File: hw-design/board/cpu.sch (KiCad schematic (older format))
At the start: 23 parts, among them P1 CHAIN, P2 USB_OTG, P3 SWD, Q7 BC857, SW1 SW_PUSH, U4 LPC11U24FBD48/401, Y1 12MHz

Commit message: sch: DRC checked
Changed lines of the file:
@@
 $EndDescr
 $Comp
-L GNDD #PWR52
+L GNDD #PWR045
 U 1 1 54E5DFA7
 P 9200 4250
-F 0 "#PWR52" H 9200 4000 60  0001 C CNN
+F 0 "#PWR045" H 9200 4000 60  0001 C CNN
 F 1 "GNDD" H 9200 4100 60  0000 C CNN
 F 2 "" H 9200 4250 60  0000 C CNN
@@
 $EndComp
 $Comp
-L GNDD #PWR43
+L GNDD #PWR046
 U 1 1 556F6417
 P 3300 4600
-F 0 "#PWR43" H 3300 4350 50  0001 C CNN
+F 0 "#PWR046" H 3300 4350 50  0001 C CNN
 F 1 "GNDD" H 3300 4450 50  0000 C CNN
 F 2 "" H 3300 4600 60  0000 C CNN
@@
 $EndComp
 $Comp
-L GNDD #PWR44
+L GNDD #PWR047
 U 1 1 556F65EC
 P 3550 4600
-F 0 "#PWR44" H 3550 4350 50  0001 C CNN
+F 0 "#PWR047" H 3550 4350 50  0001 C CNN
 F 1 "GNDD" H 3550 4450 50  0000 C CNN
 F 2 "" H 3550 4600 60  0000 C CNN
@@
 $EndComp
 $Comp
-L +3.3V #PWR49
+L +3.3V #PWR048
 U 1 1 55705A80
 P 5900 850
-F 0 "#PWR49" H 5900 700 50  0001 C CNN
+F 0 "#PWR048" H 5900 700 50  0001 C CNN
 F 1 "+3.3V" H 5900 990 50  0000 C CNN
 F 2 "" H 5900 850 60  0000 C CNN
@@
 $EndComp
 $Comp
-L GNDD #PWR48
+L GNDD #PWR049
 U 1 1 557DC875
 P 5600 1450
-F 0 "#PWR48" H 5600 1200 50  0001 C CNN
+F 0 "#PWR049" H 5600 1200 50  0001 C CNN
 F 1 "GNDD" H 5600 1300 50  0000 C CNN
 F 2 "" H 5600 1450 60  0000 C CNN
@@
 $EndComp
 $Comp
-L GNDD #PWR51
+L GNDD #PWR050
 U 1 1 557DCAD9
 P 6200 1450
-F 0 "#PWR51" H 6200 1200 50  0001 C CNN
+F 0 "#PWR050" H 6200 1200 50  0001 C CNN
 F 1 "GNDD" H 6200 1300 50  0000 C CNN
 F 2 "" H 6200 1450 60  0000 C CNN
@@
 $EndComp
 $Comp
-L GNDD #PWR50
+L GNDD #PWR051
 U 1 1 557DD01E
 P 5900 4750
-F 0 "#PWR50" H 5900 4500 50  0001 C CNN
+F 0 "#PWR051" H 5900 4500 50  0001 C CNN
 F 1 "GNDD" H 5900 4600 50  0000 C CNN
 F 2 "" H 5900 4750 60  0000 C CNN
@@
 $EndComp
 $Comp
-L GNDD #PWR42
+L GNDD #PWR052
 U 1 1 557DE7E3
 P 2850 6600
-F 0 "#PWR42" H 2850 6350 50  0001 C CNN
+F 0 "#PWR052" H 2850 6350 50  0001 C CNN
 F 1 "GNDD" H 2850 6450 50  0000 C CNN
 F 2 "" H 2850 6600 60  0000 C CNN
@@
 $EndComp
 $Comp
-L VCC #PWR45
+L VCC #PWR053
 U 1 1 557DE7F0
 P 3750 6300
-F 0 "#PWR45" H 3750 6150 50  0001 C CNN
+F 0 "#PWR053" H 3750 6150 50  0001 C CNN
 F 1 "VCC" H 3750 6450 50  0000 C CNN
 F 2 "" H 3750 6300 60  0000 C CNN
@@
 $EndComp
 $Comp
-L +3.3V #PWR41
+L +3.3V #PWR054
 U 1 1 557E22DB
 P 2050 6500
-F 0 "#PWR41" H 2050 6350 50  0001 C CNN
+F 0 "#PWR054" H 2050 6350 50  0001 C CNN
 F 1 "+3.3V" H 2050 6640 50  0000 C CNN
 F 2 "" H 2050 6500 60  0000 C CNN
@@
 $EndComp
 $Comp
-L GNDD #PWR46
+L GNDD #PWR055
 U 1 1 557EA320
 P 3750 6900
-F 0 "#PWR46" H 3750 6650 50  0001 C CNN
+F 0 "#PWR055" H 3750 6650 50  0001 C CNN
 F 1 "GNDD" H 3750 6750 50  0000 C CNN
 F 2 "" H 3750 6900 60  0000 C CNN
@@
 $EndComp
 $Comp
-L GNDD #PWR40
+L GNDD #PWR056
 U 1 1 557F3440
 P 1700 1450
-F 0 "#PWR40" H 1700 1200 50  0001 C CNN
+F 0 "#PWR056" H 1700 1200 50  0001 C CNN
 F 1 "GNDD" H 1700 1300 50  0000 C CNN
 F 2 "" H 1700 1450 60  0000 C CNN
@@
 $EndComp
 $Comp
-L +3.3V #PWR54
+L +3.3V #PWR057
 U 1 1 55802FA1
 P 10000 1250
-F 0 "#PWR54" H 10000 1100 50  0001 C CNN
+F 0 "#PWR057" H 10000 1100 50  0001 C CNN
 F 1 "+3.3V" H 10000 1390 50  0000 C CNN
 F 2 "" H 10000 1250 60  0000 C CNN
@@
 $EndComp
 $Comp
-L GNDD #PWR55
+L GNDD #PWR058
 U 1 1 55803C49
 P 10000 2250
-F 0 "#PWR55" H 10000 2000 50  0001 C CNN
+F 0 "#PWR058" H 10000 2000 50  0001 C CNN
 F 1 "GNDD" H 10000 2100 50  0000 C CNN
 F 2 "" H 10000 2250 60  0000 C CNN
@@
 $EndComp
 $Comp
-L GNDD #PWR53
+L GNDD #PWR059
 U 1 1 55806665
 P 9600 2550
-F 0 "#PWR53" H 9600 2300 50  0001 C CNN
+F 0 "#PWR059" H 9600 2300 50  0001 C CNN
 F 1 "GNDD" H 9600 2400 50  0000 C CNN
 F 2 "" H 9600 2550 60  0000 C CNN
@@
 LCD_CONTRAST
 Wire Wire Line
-	9200 3850 9200 3950
-Wire Wire Line
-	9200 3950 9200 4150
-Wire Wire Line
-	9200 4150 9200 4250
+	9200 3850 9200 4250
 Wire Wire Line
 	9900 4150 10100 4150
@@
 	4050 4100 4050 4200
 Wire Wire Line
-	4050 4200 3850 4200
-Wire Wire Line
-	3850 4200 3550 4200
+	4050 4200 3550 4200
 Wire Wire Line
 	3550 4200 3550 4250
@@
 	3300 4250 3300 3900
 Wire Wire Line
-	3300 3900 3850 3900
-Wire Wire Line
-	3850 3900 4050 3900
+	3300 3900 4050 3900
 Wire Wire Line
 	4050 3900 4050 4000
@@
 	5800 1600 5800 900
 Wire Wire Line
-	5600 900  5800 900
-Wire Wire Line
-	5800 900  5900 900
-Wire Wire Line
-	5900 900  6000 900
-Wire Wire Line
-	6000 900  6200 900
+	5600 900  6200 900
 Wire Wire Line
 	6000 900  6000 1600
@@
 	5800 4600 5800 4700
 Wire Wire Line
-	5800 4700 5900 4700
-Wire Wire Line
-	5900 4700 6000 4700
+	5800 4700 6000 4700
 Wire Wire Line
 	6000 4700 6000 4600
@@
 	3450 7200 3450 6400
 Wire Wire Line
-	4200 6450 4350 6450
-Wire Wire Line
-	4350 6450 4500 6450
-Wire Wire Line
-	3550 6450 3750 6450
-Wire Wire Line
-	3750 6450 3900 6450
+	4200 6450 4500 6450
+Wire Wire Line
+	3550 6450 3900 6450
 Wire Wire Line
 	3550 6450 3550 6400
 Wire Wire Line
-	3750 6300 3750 6450
-Wire Wire Line
-	3750 6450 3750 6550
+	3750 6300 3750 6550
 Wire Wire Line
 	2850 6100 2850 6000
 Wire Wire Line
-	2650 6000 2850 6000
-Wire Wire Line
-	2850 6000 2950 6000
+	2650 6000 2950 6000
 Wire Wire Line
 	2650 6000 2650 6100
@@
 	2650 6400 2650 6500
 Wire Wire Line
-	2650 6500 2850 6500
-Wire Wire Line
-	2850 6500 3150 6500
+	2650 6500 3150 6500
 Wire Wire Line
 	3150 6500 3150 6400
 Wire Wire Line
-	2850 6400 2850 6500
-Wire Wire Line
-	2850 6500 2850 6600
+	2850 6400 2850 6600
 Wire Wire Line
 	3950 3700 4100 3700
@@
 	4100 3800 3950 3800
 Wire Wire Line
-	1950 7100 2050 7100
-Wire Wire Line
-	2050 7100 2150 7100
+	1950 7100 2150 7100
 Wire Wire Line
 	2050 7000 2050 7100
@@
 	1650 7100 1500 7100
 Wire Wire Line
-	2050 6500 2050 6600
-Wire Wire Line
-	2050 6600 2050 6700
+	2050 6500 2050 6700
 Wire Wire Line
 	2450 6900 2450 6600
@@
 	2450 7350 2600 7350
 Wire Wire Line
-	2900 7350 3350 7350
-Wire Wire Line
-	3350 7350 3850 7350
+	2900 7350 3850 7350
 Wire Wire Line
 	3750 6900 3750 6850
@@
 	10000 1350 10000 1250
 Wire Wire Line
-	10000 1650 10000 1750
-Wire Wire Line
-	10000 1750 10000 1850
+	10000 1650 10000 1850
 Wire Wire Line
 	10000 2150 10000 2250
 Wire Wire Line
-	9350 1750 9600 1750
-Wire Wire Line
-	9600 1750 10000 1750
+	9350 1750 10000 1750
 Wire Wire Line
 	9600 1850 9600 1750
@@
 Connection ~ 4350 6450
 $Comp
-L GNDD #PWR47
+L GNDD #PWR060
 U 1 1 558C35D8
 P 4350 6900
-F 0 "#PWR47" H 4350 6650 50  0001 C CNN
+F 0 "#PWR060" H 4350 6650 50  0001 C CNN
 F 1 "GNDD" H 4350 6750 50  0000 C CNN
 F 2 "" H 4350 6900 60  0000 C CNN

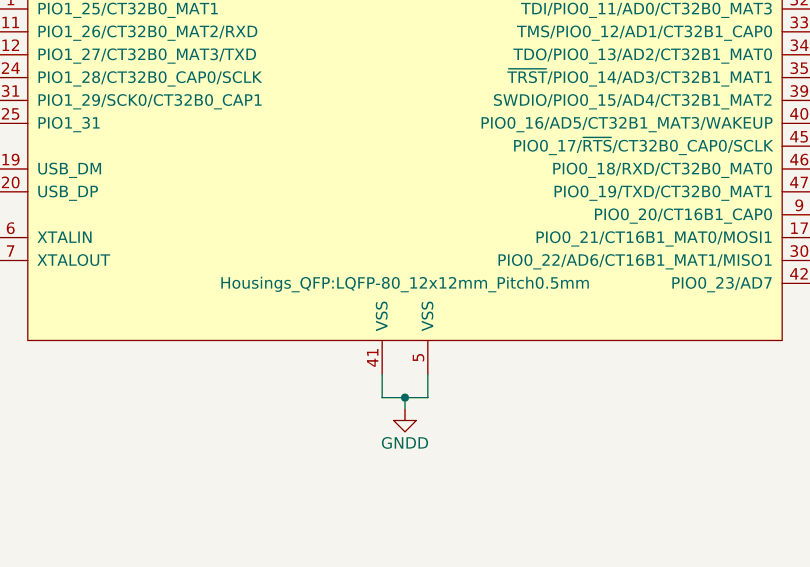
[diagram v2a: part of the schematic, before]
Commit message: sch: fixing some footprints and MPN
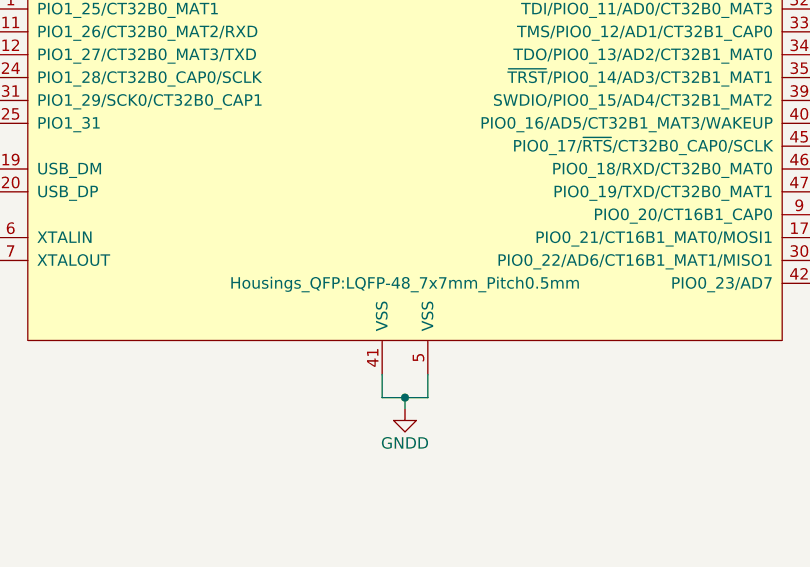
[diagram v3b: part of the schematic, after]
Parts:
- U4: footprint Housings_QFP:LQFP-80_12x12mm_Pitch0.5mm -> Housings_QFP:LQFP-48_7x7mm_Pitch0.5mm
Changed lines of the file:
@@
 F 0 "U4" H 4400 4500 50  0000 C CNN
 F 1 "LPC11U24FBD48/401" H 7100 4500 50  0000 C CNN
-F 2 "Housings_QFP:LQFP-80_12x12mm_Pitch0.5mm" H 5900 2000 50  0000 C CNN
+F 2 "Housings_QFP:LQFP-48_7x7mm_Pitch0.5mm" H 5900 2000 50  0000 C CNN
 F 3 "" H 5850 3050 60  0000 C CNN
 F 4 "LPC11U24FBD48/401" H 0   0   50  0001 C CNN "MPN"
